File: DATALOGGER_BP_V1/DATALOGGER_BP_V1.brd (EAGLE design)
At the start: 130 x 50 mm, 52 parts, among them J1 1985247, J2 1985247, J3 1985247, J4 1985247, J5 1985247, J6 1985247, J7 1985247, J8 1985247, J9 1755736

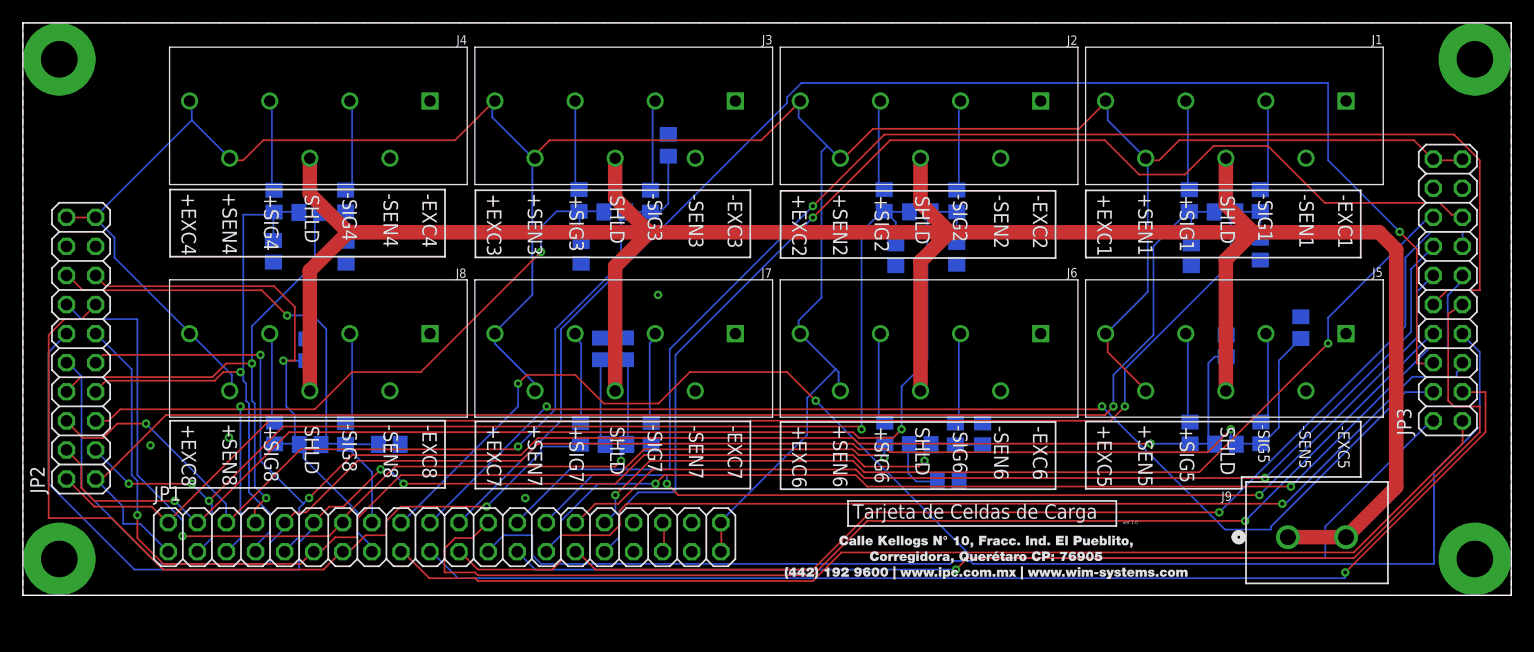
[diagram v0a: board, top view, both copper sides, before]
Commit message: tarjeta_v18
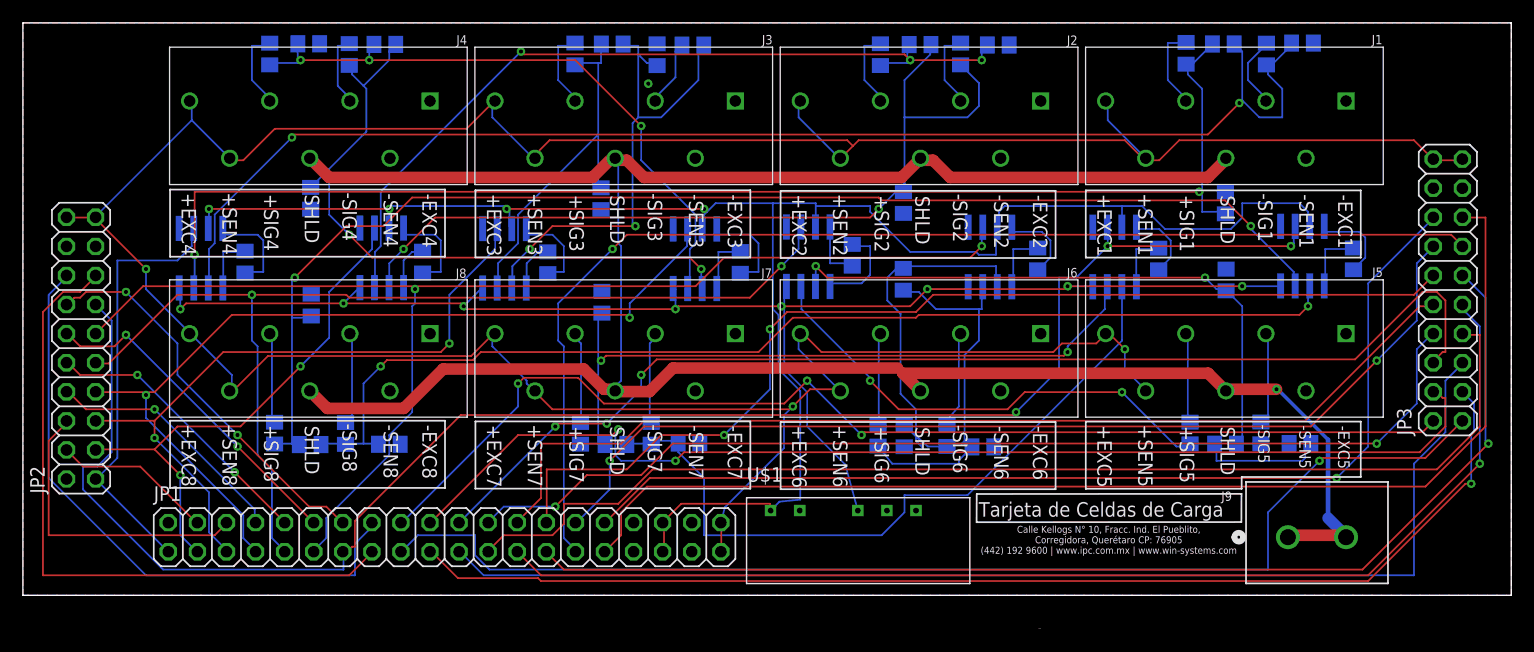
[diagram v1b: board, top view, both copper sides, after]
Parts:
- added IC1, IC2, IC3, IC4, IC5, IC6, IC7, IC8: AD620R, analog-devices:SO8
- added R17, R18, R19, R20, R21, R22, R23, R24: 34.8, rcl:R0805
- added U$1: TMH2412D, TMH 2412D:TMH2412D
- moved C12 20.4 mm to (85.2, 48.1), turned to 180 degrees
- moved C16 18.4 mm to (25.0, 48.2), turned to 180 degrees
- moved C9 18.4 mm to (111.8, 48.2), turned to 180 degrees
- moved C4 16.1 mm to (31.6, 48.1)
- moved C1 14.7 mm to (104.8, 48.2)
- moved C3 14.7 mm to (51.5, 48.1)
- moved C2 14.6 mm to (78.4, 48.1)
- moved C6 14.5 mm to (76.9, 27.6), turned to 270 degrees
- moved R5 14.1 mm to (58.5, 48.1), turned to 0 degrees
- moved R2 12.9 mm to (101.6, 47.3)
- moved R8 12.9 mm to (21.6, 47.3)
- moved R3 12.8 mm to (81.9, 47.3)
- moved R1 12.8 mm to (108.6, 47.3)
- moved R6 12.8 mm to (48.2, 47.3)
- moved R7 12.8 mm to (28.5, 47.2)
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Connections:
- new net -12V: IC1.4, IC2.4, IC3.4, IC4.4, IC5.4, IC6.4, IC7.4, IC8.4, U$1.P$3
- new net N$17: IC1.8, R17.1
- new net N$18: IC1.1, R17.2
- new net N$19: IC3.1, R19.2
- new net N$20: IC3.8, R19.1
- new net N$21: IC2.1, R18.2
- new net N$22: IC2.8, R18.1
- new net N$23: IC4.8, R20.1
- new net N$24: IC4.1, R20.2
- new net N$25: IC5.8, R21.1
- new net N$26: IC5.1, R21.2
- new net N$27: IC6.1, R22.2
- new net N$28: IC6.8, R22.1
- new net N$29: IC7.1, R23.2
- new net N$30: IC7.8, R23.1
- new net N$33: IC8.8, R24.1
- new net N$34: IC8.1, R24.2
- new net SIG1+: C1.2, C10.1, IC1.3, R2.1
- new net SIG1-: C1.1, C9.1, IC1.2, R1.1
- new net SIG2+: C12.1, C2.2, IC2.3, R4.1
- new net SIG2-: C11.1, C2.1, IC2.2, R3.1
- new net SIG3+: C14.1, C3.2, IC3.3, R6.1
- new net SIG3-: C13.1, C3.1, IC3.2, R5.1
- new net SIG4+: C16.1, C4.2, IC4.3, R8.1
- new net SIG4-: C15.1, C4.1, IC4.2, R7.1
- new net SIG5+: C18.1, C5.2, IC5.3, R10.1
- new net SIG5-: C17.1, C5.1, IC5.2, R9.1
- new net SIG6+: C20.1, C6.2, IC6.3, R12.1
- new net SIG6-: C19.1, C6.1, IC6.2, R11.1
- new net SIG7+: C22.1, C7.2, IC7.3, R14.1
- new net SIG7-: C21.1, C7.1, IC7.2, R13.1
- new net SIG8+: C24.1, C8.2, IC8.3, R16.1
- new net SIG8-: C23.1, C8.1, IC8.2, R15.1
- net +12V: now also IC1.7, IC2.7, IC3.7, IC4.7, IC5.7, IC6.7, IC7.7, IC8.7, U$1.P$1
- net GND: now also IC1.5, IC2.5, IC3.5, IC4.5, IC5.5, IC6.5, IC7.5, IC8.5, JP1.2, U$1.P$2, U$1.P$4
- net INPUT1+: now also IC1.6; no longer C1.2, C10.1, R2.1
- net INPUT1-: no longer C1.1, C9.1, JP1.2, R1.1
- net INPUT2+: now also IC2.6; no longer C12.1, C2.2, R4.1
- net INPUT2-: no longer C11.1, C2.1, R3.1
- net INPUT3+: now also IC3.6; no longer C14.1, C3.2, R6.1
- net INPUT3-: no longer C13.1, C3.1, R5.1
- net INPUT4+: now also IC4.6; no longer C16.1, C4.2, R8.1
- net INPUT4-: no longer C15.1, C4.1, R7.1
- net INPUT5+: now also IC5.6; no longer C18.1, C5.2, R10.1
- net INPUT5-: no longer C17.1, C5.1, R9.1
- net INPUT6+: now also IC6.6; no longer C20.1, C6.2, R12.1
- net INPUT6-: no longer C19.1, C6.1, R11.1
- net INPUT7+: now also IC7.6, IC8.6; no longer C22.1, C7.2, R14.1
- net INPUT7-: no longer C21.1, C7.1, R13.1
- net INPUT8+: no longer C24.1, C8.2, R16.1
- net INPUT8-: no longer C23.1, C8.1, R15.1
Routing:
- net +12V: track 2.63 -> 160.8 mm, vias 0 -> 4
- net -12V: track 0.00 -> 133.7 mm, vias 0 -> 8
- net INPUT1-: track 123.7 -> 0.00 mm, vias 1 -> 0
- net SIG1-: track 0.00 -> 118.5 mm, vias 0 -> 2
- net SIG1+: track 0.00 -> 115.5 mm, vias 0 -> 2
- net SIG8+: track 0.00 -> 113.4 mm, vias 0 -> 2
- net INPUT5-: track 136.0 -> 24.8 mm, vias 1 -> 2
- net SIG8-: track 0.00 -> 97.5 mm, vias 0 -> 2
- net INPUT2-: track 105.6 -> 14.0 mm, vias 2 -> 0
- net INPUT1+: track 126.4 -> 37.6 mm, vias 1 -> 0
- net INPUT6-: track 107.0 -> 29.2 mm, vias 3 -> 2
- net SIG2-: track 0.00 -> 75.0 mm, vias 0 -> 2
- net SIG2+: track 0.00 -> 72.5 mm, vias 0 -> 3
- net INPUT7+: track 84.8 -> 149.2 mm, vias 1 -> 3
- net SIG7-: track 0.00 -> 63.0 mm
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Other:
- board text added: "Calle Kellogs N° 10, Fracc. Ind. El Pueblito, Corregidora, Querétaro CP: 76905 (442) 192 9600 | www.ipc.com.mx | www.win-systems.com"
- board text removed: "ver 1.0"
